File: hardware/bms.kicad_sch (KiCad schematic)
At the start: 15 parts

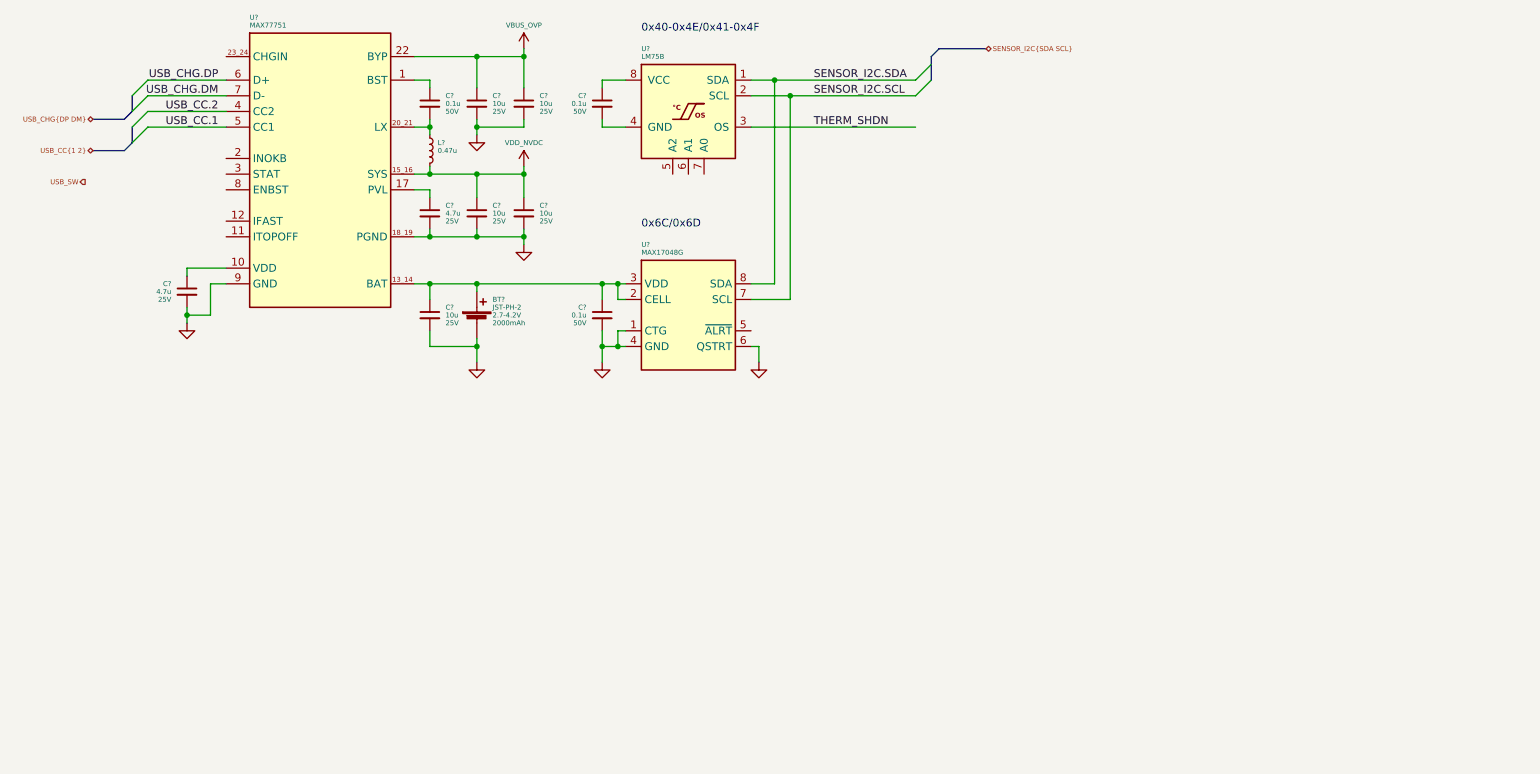
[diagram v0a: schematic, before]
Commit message: usb, charger, sensors, heir
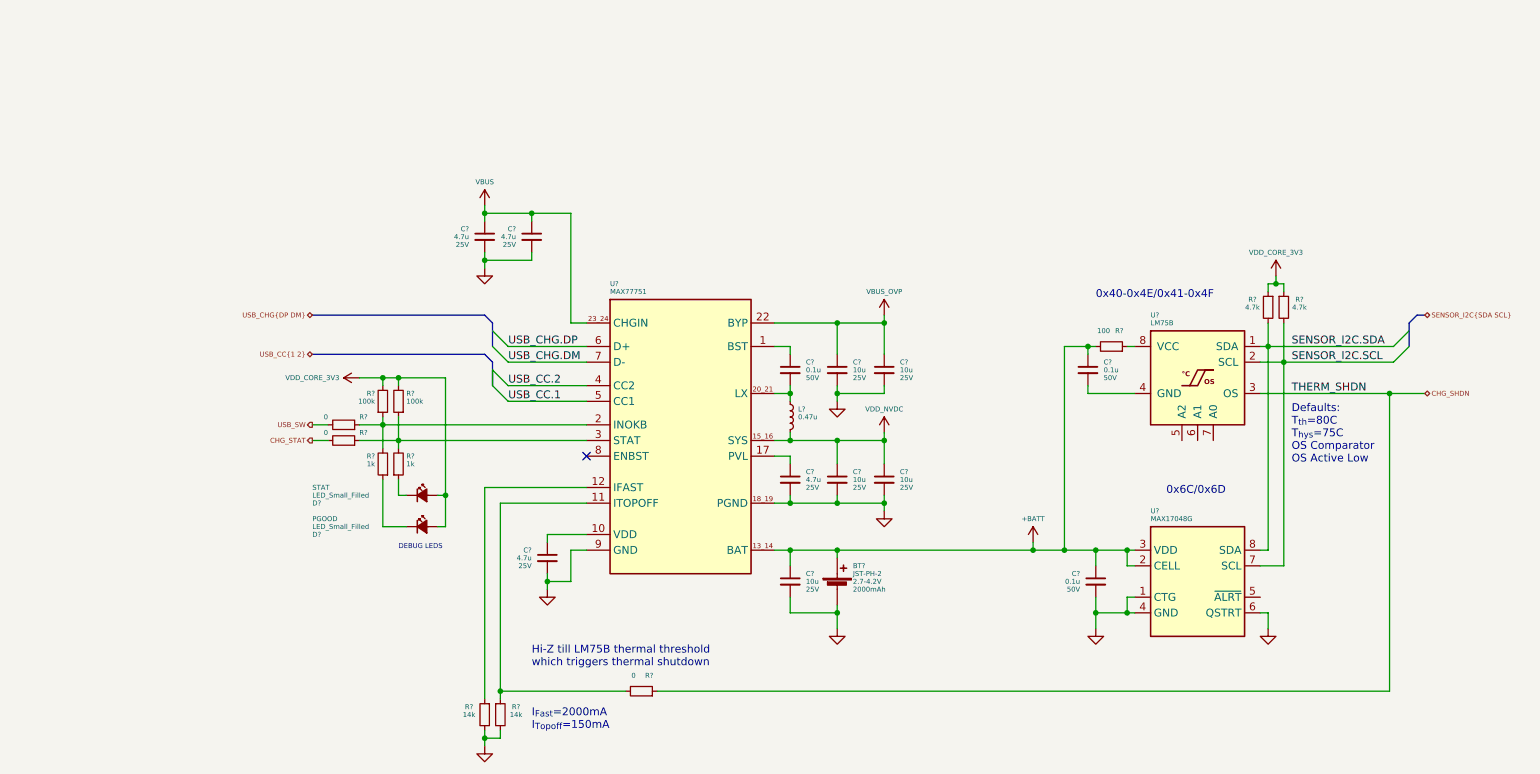
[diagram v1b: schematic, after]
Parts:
- added C? (x2): 4.7u, Capacitor_SMD:C_0805_2012Metric, symbol Device:C_Small
- added D? (x2): LED_Small_Filled, symbol Device:LED_Small_Filled
- added R? (x2): 100k, Resistor_SMD:R_0603_1608Metric, symbol Device:R_Small
- added R? (x2): 1k, Resistor_SMD:R_0603_1608Metric, symbol Device:R_Small
- added R? (x3): 0, Resistor_SMD:R_0603_1608Metric, symbol Device:R_Small
- added R?: 100, Resistor_SMD:R_0603_1608Metric, symbol Device:R_Small
- added R? (x2): 14k, Resistor_SMD:R_0603_1608Metric, symbol Device:R_Small
- added R? (x2): 4.7k, Resistor_SMD:R_0603_1608Metric, symbol Device:R_Small
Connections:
- net GND: now also C?.2, C?.2, R?.2, R?.2
- net SENSOR_I2C.SCL: now also R?.2
- net SENSOR_I2C.SDA: now also R?.2
- net USB_SW: now also R?.2
- net +BATT: now reaches BT?.1 (+), C?.1, C?.1, U?.13_14 (BAT), U?.2 (CELL), U?.3 (VDD)
- net +BATT: now also C?.1, R?.2
- net at U?.11 (ITOPOFF): now also R?.1, R?.2
- net at U?.12 (IFAST): now also R?.1
- net at U?.2 (INOKB): now also R?.1, R?.1, R?.2
- net VBUS: now reaches U?.23_24 (CHGIN)
- net VBUS: now also C?.1, C?.1
- net at U?.3 (STAT): now also R?.1, R?.1, R?.2
- net at U?.8 (VCC): now also R?.1; no longer C?.1
- net THERM_SHDN renamed CHG_SHDN
- net CHG_SHDN: now also R?.1
- new net: D?.1 (K), R?.1 (x2)
- new net 3V3_CORE: D?.2 (A), D?.2 (A), R?.1, R?.1, R?.2, R?.2
- new net CHG_STAT: R?.2
- no-connect marks 0 -> 1
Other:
- note added: "DEBUG LEDS"
- note added: "Defaults: T_{th}=80C T_{hys}=75C OS Comparator OS Active Low"
- note added: "Hi-Z till LM75B thermal threshold which triggers thermal shutdown"
- note added: "I_{Fast}=2000mA I_{Topoff}=150mA"
- moved on the sheet: BT?, C?, L?, U?
